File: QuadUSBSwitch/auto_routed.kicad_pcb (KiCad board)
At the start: 2 copper layers, 15 parts, among them J1 USB_A, J2 USB_A, J3 USB_OTG, J4 USB_OTG, J5 USB_OTG, J6 USB_OTG, J7 USB_OTG, SW1 SW_DIP_x04, U1 CH440G

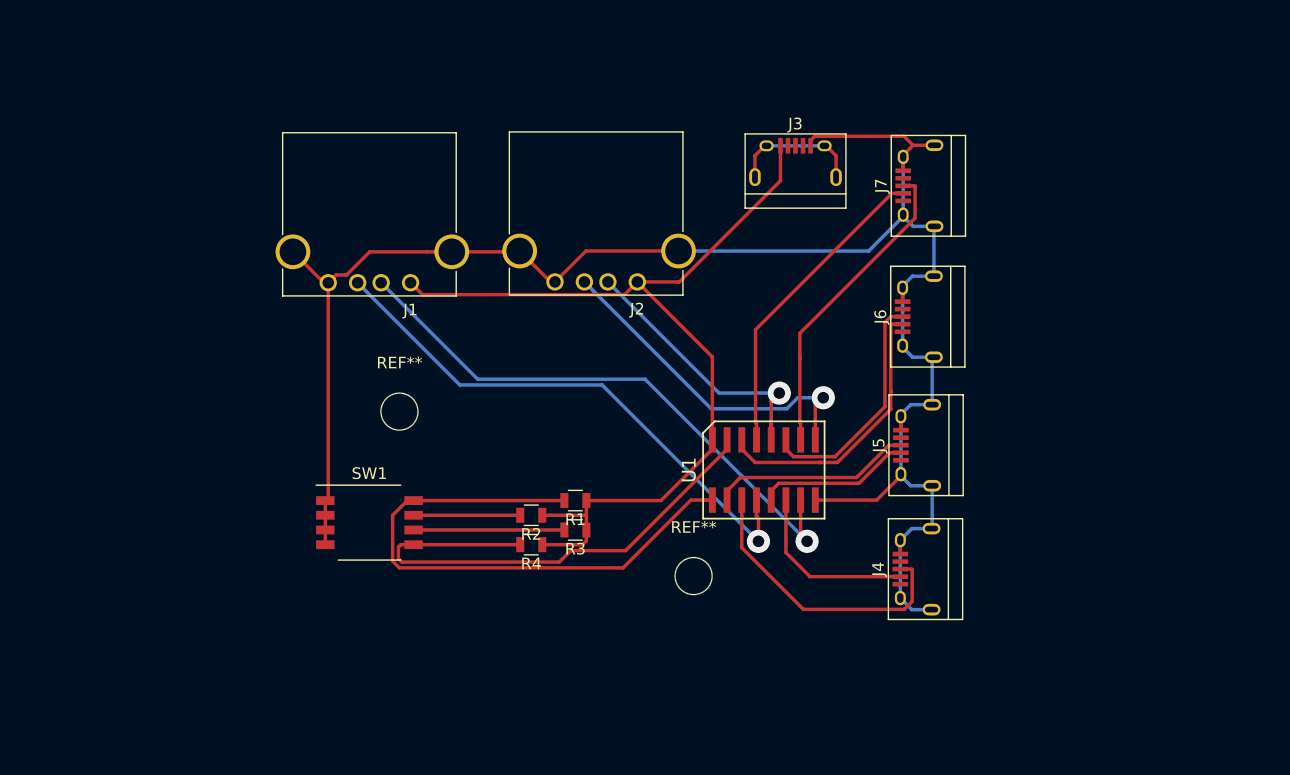
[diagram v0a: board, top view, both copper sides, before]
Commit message: update; a test dual layer one is ready
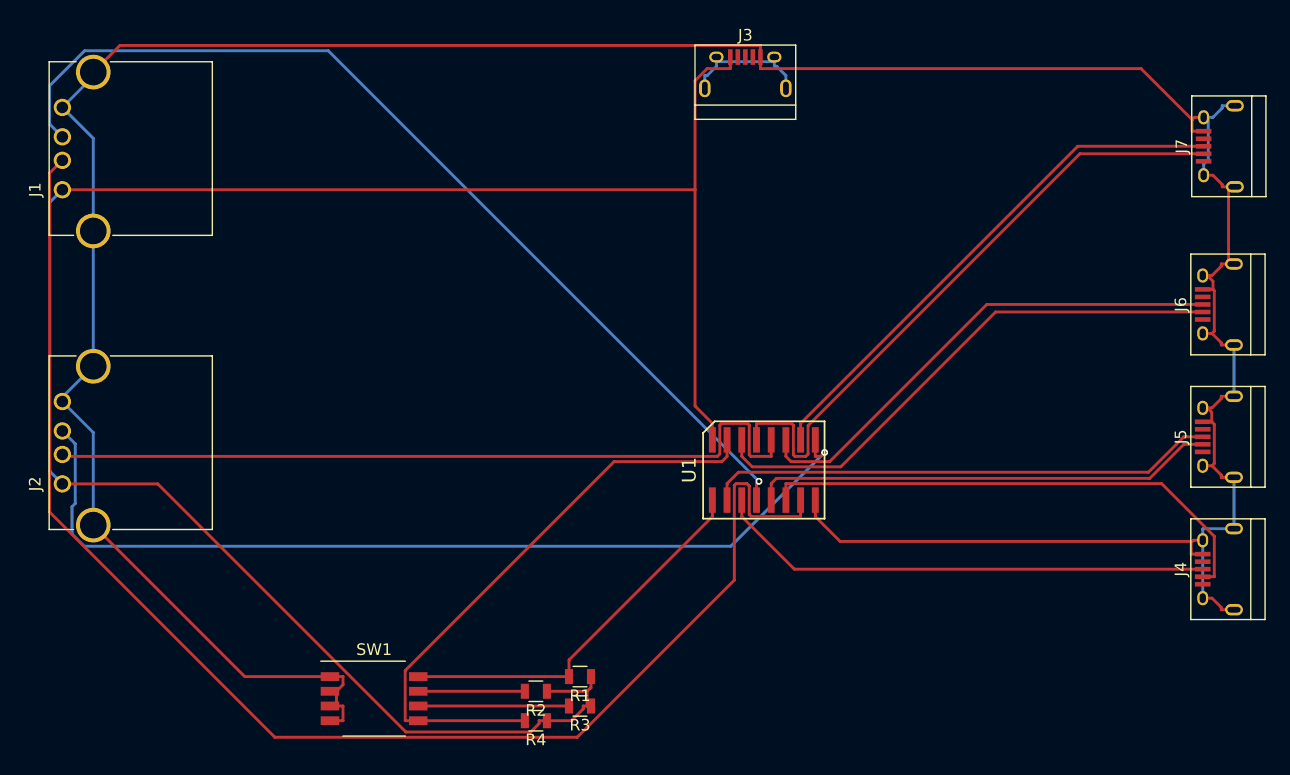
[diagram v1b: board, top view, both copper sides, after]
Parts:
- removed REF** (x2): MountingHole_3.2mm_M3, Mounting_Holes:MountingHole_3.2mm_M3
- moved J2 52.6 mm to (53.1, 90.0), turned to 90 degrees
- moved J1 31.1 mm to (53.1, 64.6), turned to 90 degrees
- moved J7 26.2 mm to (153.0, 60.9)
- moved J4 26.1 mm to (152.9, 97.4)
- moved J5 26.1 mm to (152.9, 86.0)
- moved J6 25.9 mm to (152.9, 74.5)
- moved R1 15.2 mm to (97.8, 106.7)
- moved R2 15.2 mm to (94.0, 108.0)
- moved R3 15.2 mm to (97.8, 109.2)
- moved R4 15.2 mm to (94.0, 110.5)
- moved SW1 15.2 mm to (80.0, 108.6)
- moved J3 8.81 mm to (112.1, 54.5)
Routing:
- net GND: track 162.1 -> 282.3 mm
- net VBUS: track 80.8 -> 179.0 mm
- net Net-(J1-Pad2): track 49.9 -> 121.6 mm, vias 1 -> 0
- net Net-(J2-Pad3): track 29.5 -> 80.6 mm
- net Net-(J2-Pad2): track 24.5 -> 68.0 mm, vias 1 -> 0
- net Net-(J1-Pad3): track 47.5 -> 84.5 mm
- net Net-(J4-Pad2): track 16.1 -> 44.8 mm
- net Net-(J7-Pad2): track 27.2 -> 55.0 mm
- net Net-(J5-Pad3): track 17.4 -> 44.2 mm
- net Net-(J5-Pad2): track 13.4 -> 40.1 mm
- net Net-(J6-Pad3): track 20.4 -> 43.2 mm
- net Net-(J6-Pad2): track 24.8 -> 47.1 mm
- net Net-(J7-Pad3): track 27.2 -> 46.1 mm
- net Net-(J4-Pad3): track 25.1 -> 43.1 mm
- net Net-(R1-Pad2): track 49.6 -> 33.4 mm
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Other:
- net class testing removed
